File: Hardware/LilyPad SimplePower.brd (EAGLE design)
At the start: 28.4 x 28.4 mm, 21 parts, among them U1 MCP73831

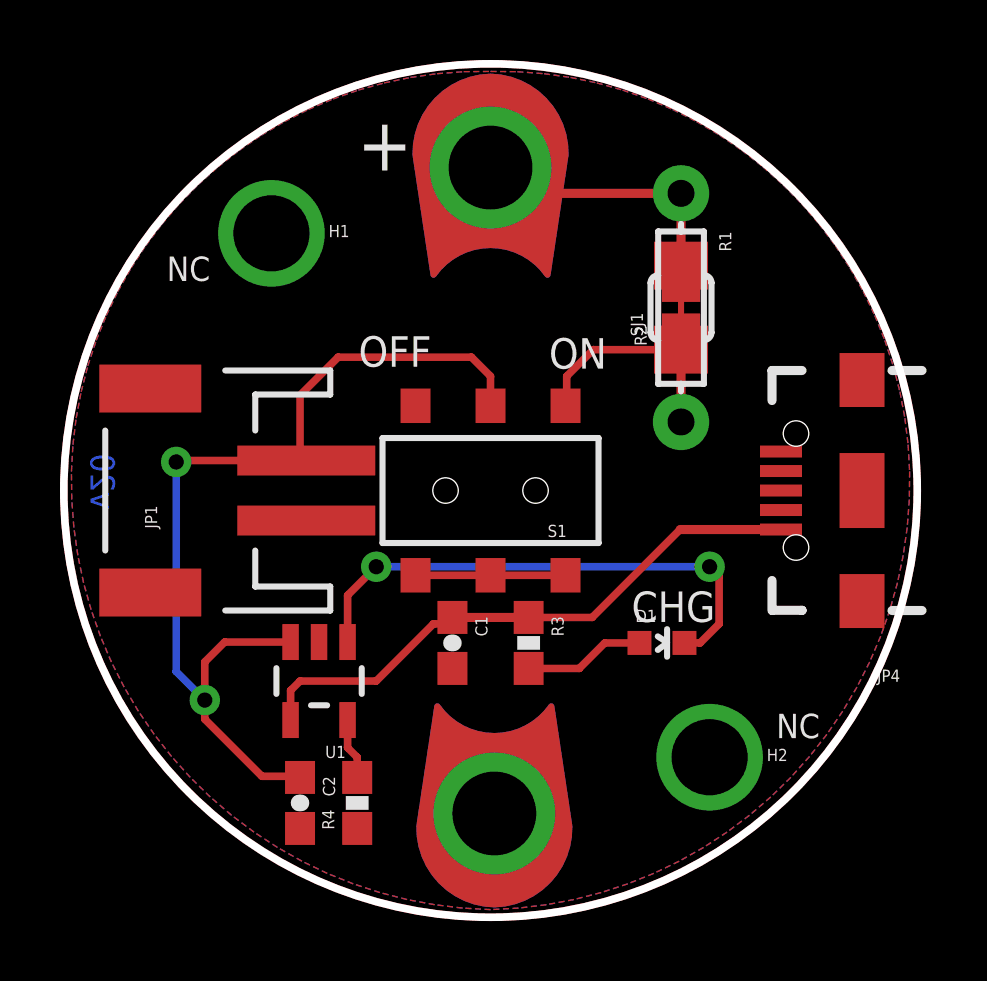
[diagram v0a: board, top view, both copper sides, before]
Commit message: midway work  on updating design
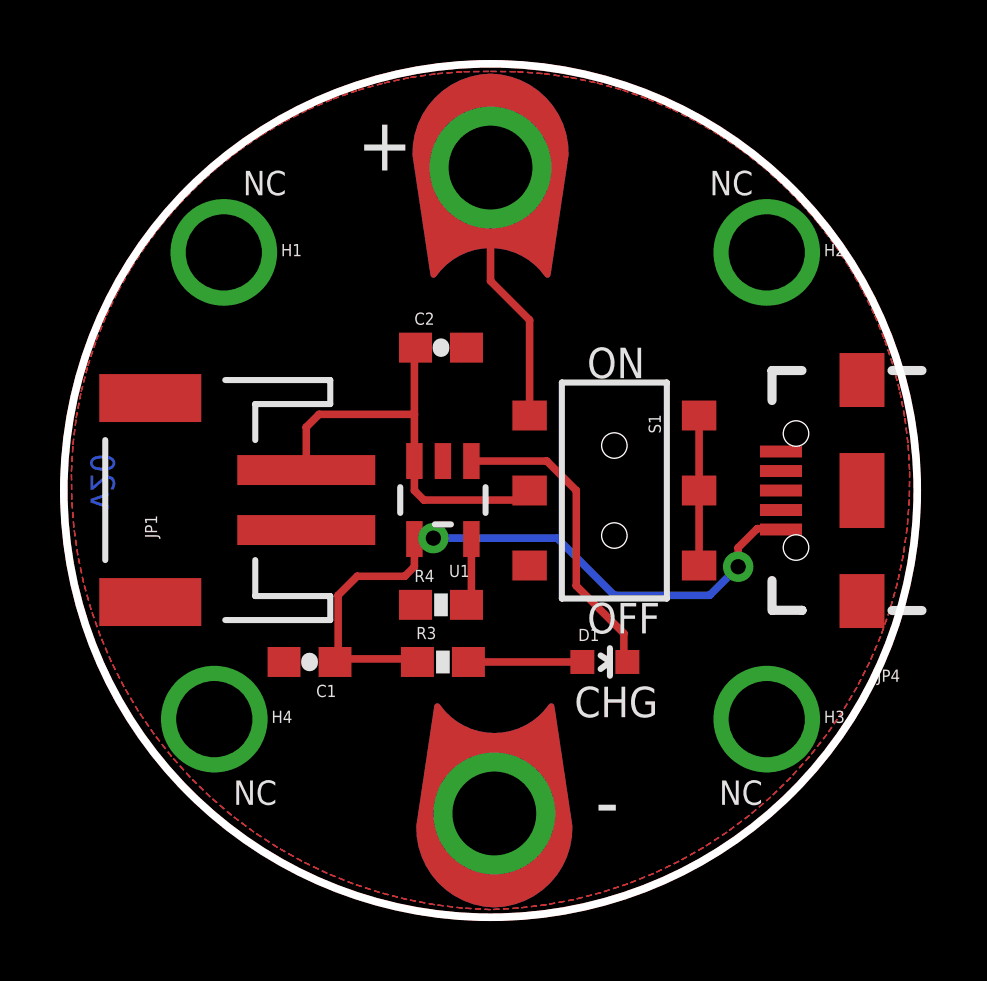
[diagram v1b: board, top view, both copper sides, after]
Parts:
- removed R1: (no value), SparkFun:AXIAL-0.3
- removed R2: (no value), SparkFun:1206
- removed SJ1: SOLDERJUMPERTRACE, SparkFun-Passives:SJ_2S-TRACE
- added H3, H4: SEW_HOLE, LilyPad-Wearables:SIMPLE_HOLE
- moved H2 16.9 mm to (9.21, 5.40)
- moved C2 15.9 mm to (-1.65, 2.22), turned to 0 degrees
- moved U1 7.31 mm to (-1.59, -2.86)
- moved R4 7.17 mm to (-1.65, -6.35), turned to 0 degrees
- moved C1 4.80 mm to (-6.03, -8.26), turned to 180 degrees
- moved S1 4.13 mm to (4.13, -2.54), turned to 270 degrees
- moved R3 2.93 mm to (-1.59, -8.26), turned to 0 degrees
- moved D1 2.01 mm to (3.81, -8.26)
- moved H1 1.71 mm to (-8.89, 5.40)
- moved U$1 1.00 mm to (0.32, 2.22)
- moved JP1 0.32 mm to (-9.84, -2.86)
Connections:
- removed net +: R1.P$1, R2.2, SJ1.2, U$4.1
- removed net N$2: R1.P$2, R2.1, S1.4, SJ1.1
- removed net SINK2: S1.6
- new net N$6: S1.4, U$4.1
- net GND: now also S1.6
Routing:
- net N$1: track 32.1 -> 14.1 mm, vias 2 -> 0
- net +: track 10.0 -> 0.00 mm
- net N$6: track 0.00 -> 8.80 mm
- net N$2: track 8.48 -> 0.00 mm
- net N$4: track 17.5 -> 10.3 mm, vias 2 -> 0
- net N$3: track 19.6 -> 23.1 mm, vias 0 -> 2
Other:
- board text added: "-"
